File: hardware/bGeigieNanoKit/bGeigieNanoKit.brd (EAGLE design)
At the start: 96.2 x 66.7 mm, 35 parts, among them T1 2SC1815

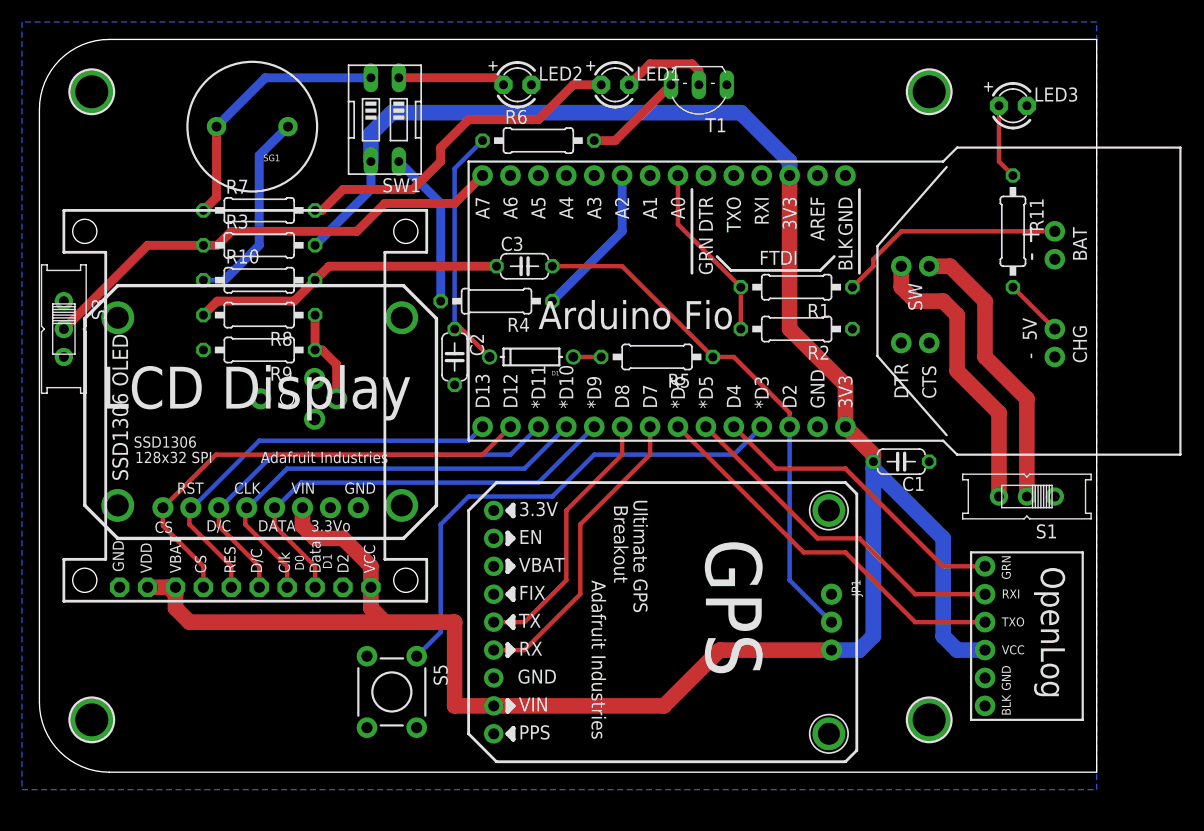
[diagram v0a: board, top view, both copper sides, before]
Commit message: cleaning up libs and updating brd
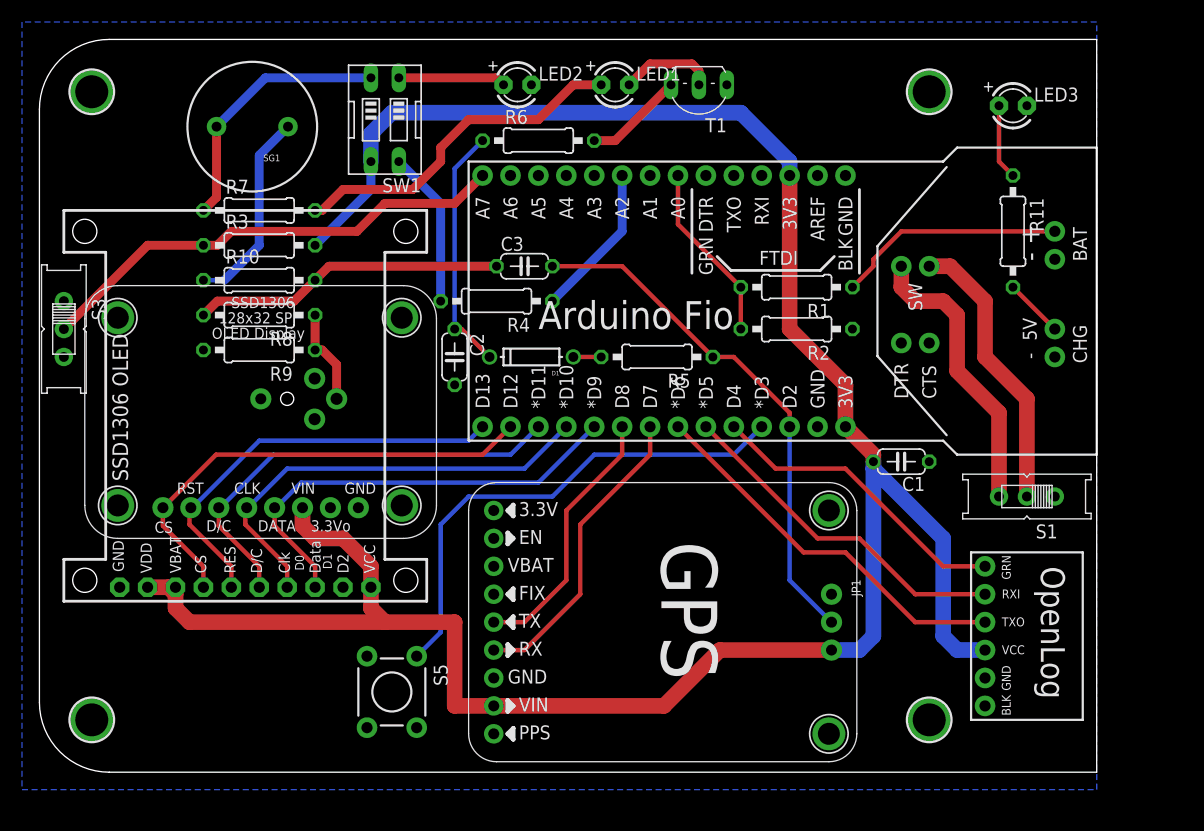
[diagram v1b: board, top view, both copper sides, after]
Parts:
- U$3: device open_hw_sockets:ULTIMATE_GPS_V3 -> open_hw_sockets:ULTIMATE_GPS_V3_TOP
- U$4: device open_hw_sockets:SSD1306_128X32_SPI_LCD -> open_hw_sockets:SSD1306_128X32_SPI_LCD_TOP
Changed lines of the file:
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@@
 </autorouter>
 <elements>
-<element name="U$4" library="open_hw_sockets" package="SSD1306_128X32_SPI_LCD" value="LCD" x="5.715" y="22.86"/>
-<element name="U$3" library="open_hw_sockets" package="ULTIMATE_GPS_V3" value="GPS" x="40.64" y="27.94" rot="R270"/>
+<element name="U$4" library="open_hw_sockets" package="SSD1306_128X32_SPI_LCD_TOP" value="LCD" x="5.715" y="22.86"/>
+<element name="U$3" library="open_hw_sockets" package="ULTIMATE_GPS_V3_TOP" value="GPS" x="40.64" y="27.94" rot="R270"/>
 <element name="LED1" library="adafruit" package="LED3MM" value="" x="53.975" y="64.135"/>
 <element name="LED2" library="adafruit" package="LED3MM" value="RED" x="45.085" y="64.135"/>
